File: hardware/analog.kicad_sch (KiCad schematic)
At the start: 1 part, among them U1 LM324

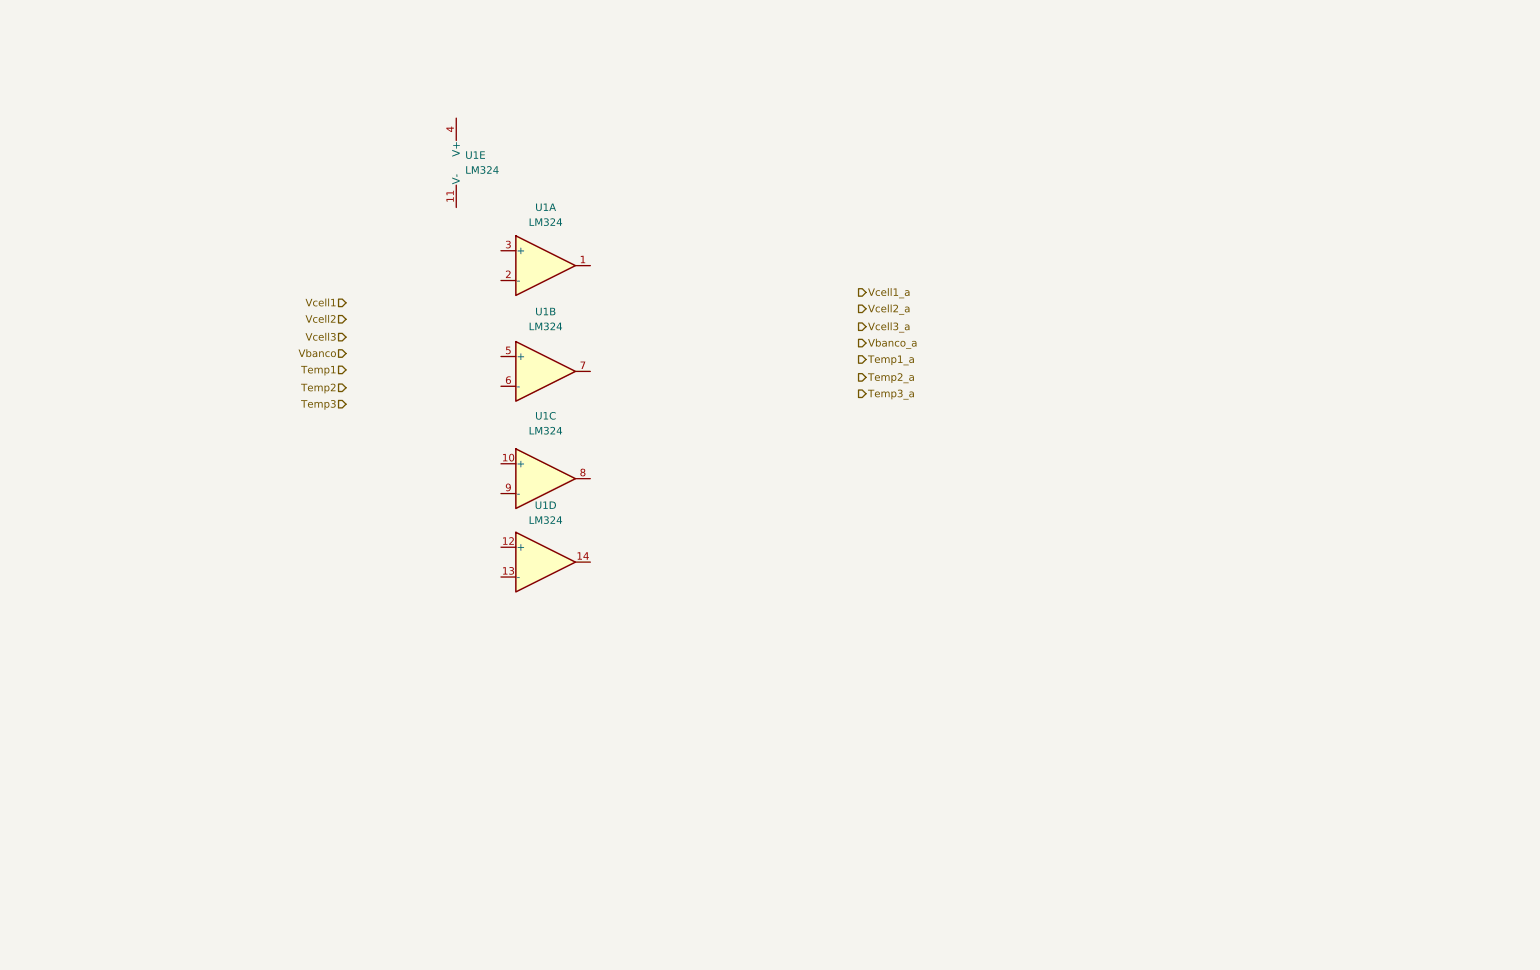
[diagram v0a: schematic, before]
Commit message: Atualização analog
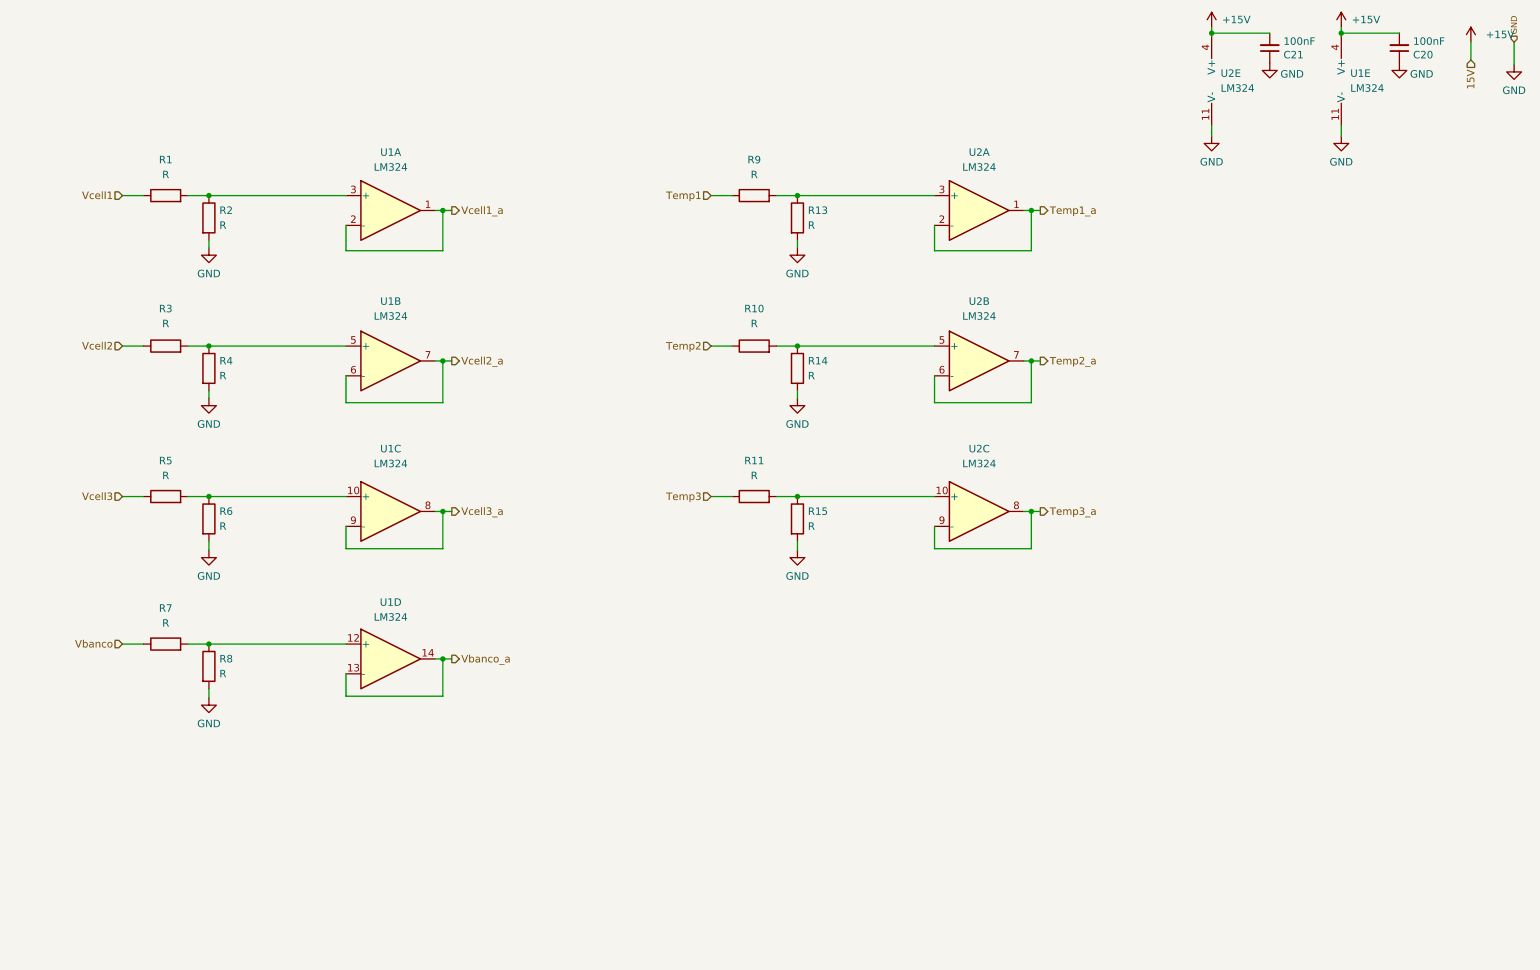
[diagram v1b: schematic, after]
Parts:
- added C20, C21: 100nF, Capacitor_SMD:C_0805_2012Metric_Pad1.18x1.45mm_HandSolder, symbol Device:C_Small
- added R1, R10, R11, R13, R14, R15, R2, R3, R4, R5, R6, R7, R8, R9: R, symbol Device:R
- added U2: LM324, symbol Amplifier_Operational:LM324
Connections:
- net Temp1: now also R9.1
- net Temp1_a: now also U2.1, U2.2 (-)
- net Temp2: now also R10.1
- net Temp2_a: now also U2.6 (-), U2.7
- net Temp3: now also R11.1
- net Temp3_a: now also U2.8, U2.9 (-)
- net Vbanco: now also R7.1
- net Vbanco_a: now also U1.13 (-), U1.14
- net Vcell1: now also R1.1
- net Vcell1_a: now also U1.1, U1.2 (-)
- net Vcell2: now also R3.1
- net Vcell2_a: now also U1.6 (-), U1.7
- net Vcell3: now also R5.1
- net Vcell3_a: now also U1.8, U1.9 (-)
- net at U1.12 (+): now also R7.2, R8.1
- net at U1.5 (+): now also R3.2, R4.1
- net at U1.3 (+): now also R1.2, R2.1
- net at U1.10 (+): now also R5.2, R6.1
- net GND: now reaches U1.11 (V-)
- net GND: now also C20.1, C21.1, R13.2, R14.2, R15.2, R2.2, R4.2, R6.2, R8.2, U2.11 (V-)
- net +15V: now reaches U1.4 (V+)
- net +15V: now also C20.2, C21.2, U2.4 (V+)
- new net: R13.1, R9.2, U2.3 (+)
- new net: R11.2, R15.1, U2.10 (+)
- new net: R10.2, R14.1, U2.5 (+)
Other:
- moved on the sheet: U1A, U1B, U1C, U1D, U1E

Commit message: Atualização analog
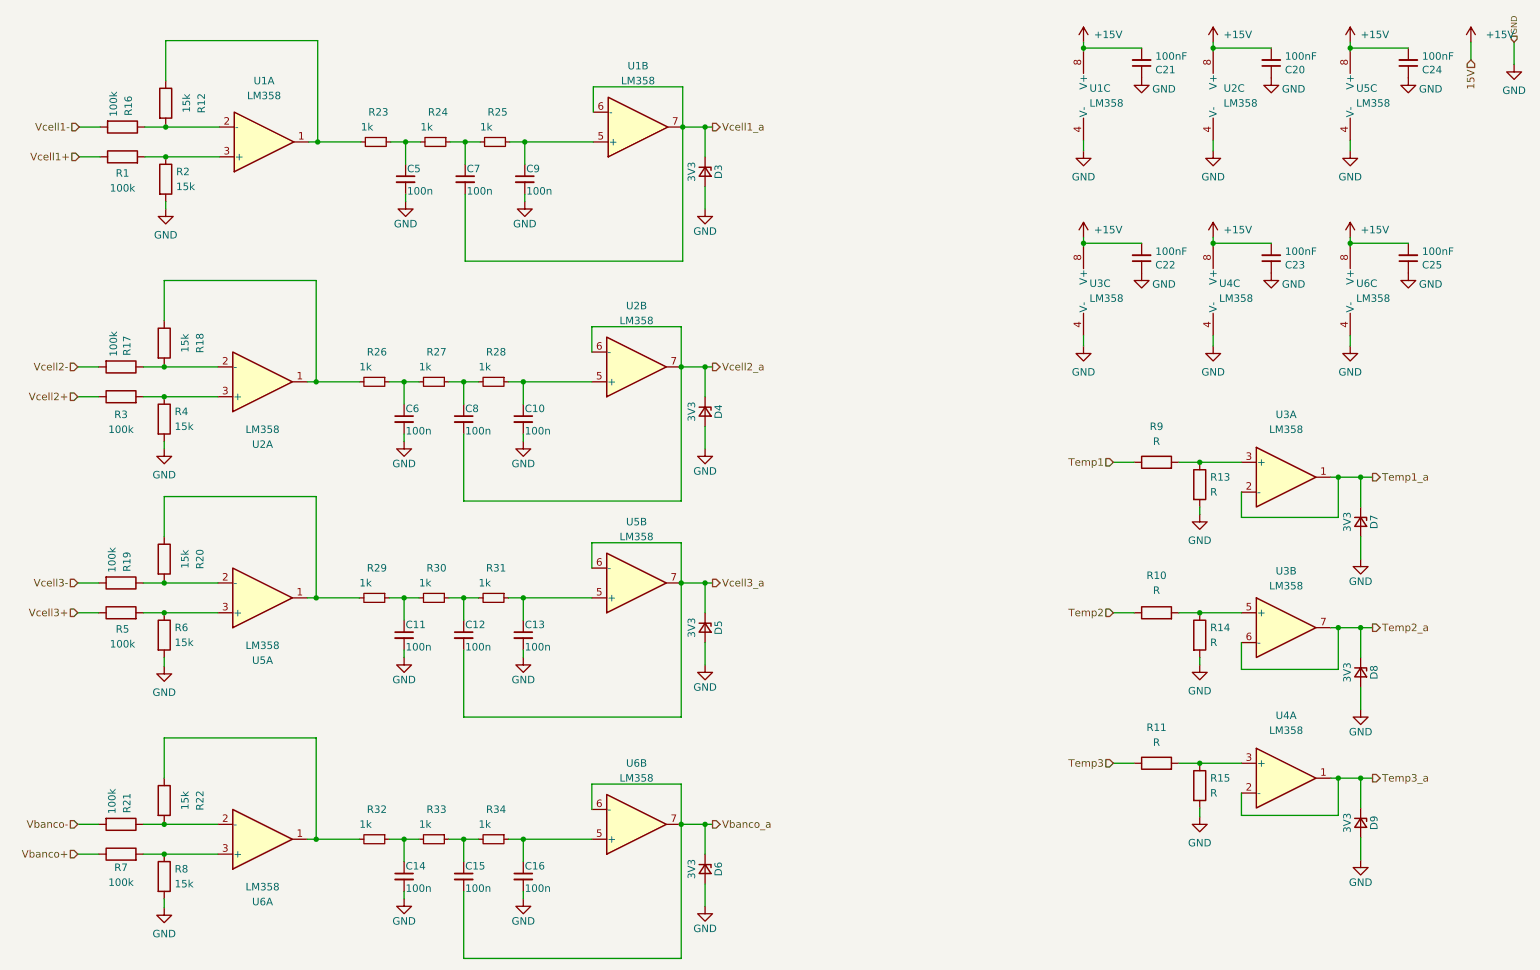
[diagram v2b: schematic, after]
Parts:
- removed U1, U2: LM324, symbol Amplifier_Operational:LM324
- added C10, C11, C12, C13, C14, C15, C16, C5, C6, C7, C8, C9: 100n, Capacitor_SMD:C_0805_2012Metric_Pad1.18x1.45mm_HandSolder, symbol Módulo-temperatura-rescue:C_Small-Device
- added C22, C23, C24, C25: 100nF, Capacitor_SMD:C_0805_2012Metric_Pad1.18x1.45mm_HandSolder, symbol Device:C_Small
- added D3, D4, D5, D6, D7, D8, D9: 3V3, Diode_SMD:D_MiniMELF_Handsoldering, symbol Módulo-temperatura-rescue:D_Zener_Small-Device
- added R12, R18, R20, R22: 15k, symbol Device:R
- added R16, R17, R19, R21: 100k, symbol Device:R
- added R23, R24, R25, R26, R27, R28, R29, R30, R31, R32, R33, R34: 1k, Resistor_SMD:R_0805_2012Metric_Pad1.20x1.40mm_HandSolder, symbol Módulo-temperatura-rescue:R_Small-Device
- added U1, U2, U3, U4, U5, U6: LM358, symbol Amplifier_Operational:LM358
- R1, R3, R5, R7: value R -> 100k
- R2, R4, R6, R8: value R -> 15k
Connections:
- net +15V: now also C22.2, C23.2, C24.2, C25.2, U1.8 (V+), U2.8 (V+), U3.8 (V+), U4.8 (V+), U5.8 (V+), U6.8 (V+)
- net GND: now also C10.2, C11.2, C13.2, C14.2, C16.2, C22.1, C23.1, C24.1, C25.1, C5.2, C6.2, C9.2, D3.2 (A), D4.2 (A), D5.2 (A), D6.2 (A), D7.2 (A), D8.2 (A), D9.2 (A), U1.4 (V-), U2.4 (V-), U3.4 (V-), U4.4 (V-), U5.4 (V-), U6.4 (V-)
- net Temp1_a: now also D7.1 (K), U3.1, U3.2 (-)
- net Temp2_a: now also D8.1 (K), U3.6 (-), U3.7
- net Temp3_a: now also D9.1 (K), U4.1, U4.2 (-)
- net Vbanco_a: now also C15.2, D6.1 (K), U6.6 (-), U6.7
- net Vcell1_a: now also C7.2, D3.1 (K), U1.6 (-), U1.7
- net Vcell2_a: now also C8.2, D4.1 (K), U2.6 (-), U2.7
- net Vcell3_a: now also C12.2, D5.1 (K), U5.6 (-), U5.7
- net at R13.1, R9.2: now also U3.3 (+)
- net at R7.2, R8.1: now also U6.3 (+)
- net at R3.2, R4.1: now also U2.3 (+)
- net at R5.2, R6.1: now also U5.3 (+)
- net at R11.2, R15.1: now also U4.3 (+)
- net at R1.2, R2.1: now also U1.3 (+)
- net at R10.2, R14.1: now also U3.5 (+)
- net Vbanco renamed Vbanco+
- net Vcell1 renamed Vcell1+
- net Vcell2 renamed Vcell2+
- net Vcell3 renamed Vcell3+
- new net: C8.1, R27.1, R28.2
- new net: C6.1, R26.1, R27.2
- new net: C10.1, R28.1, U2.5 (+)
- new net: C9.1, R25.1, U1.5 (+)
- new net: C7.1, R24.1, R25.2
- new net: C15.1, R33.1, R34.2
- new net: C14.1, R32.1, R33.2
- new net: R22.1, R32.2, U6.1
- new net: R21.1, R22.2, U6.2 (-)
- new net: R12.2, R16.1, U1.2 (-)
- new net: R17.1, R18.2, U2.2 (-)
- new net: C13.1, R31.1, U5.5 (+)
- new net: R19.1, R20.2, U5.2 (-)
- new net: R18.1, R26.2, U2.1
- new net: C5.1, R23.1, R24.2
- new net: R12.1, R23.2, U1.1
- new net: C11.1, R29.1, R30.2
- new net: R20.1, R29.2, U5.1
- new net: C12.1, R30.1, R31.2
- new net: C16.1, R34.1, U6.5 (+)
- new net Vbanco-: R21.2
- new net Vcell1-: R16.2
- new net Vcell2-: R17.2
- new net Vcell3-: R19.2
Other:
- moved on the sheet: C20, C21, R1, R10, R11, R13, R14, R15, R2, R3, R4, R5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
